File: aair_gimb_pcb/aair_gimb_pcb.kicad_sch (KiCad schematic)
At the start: 0 parts

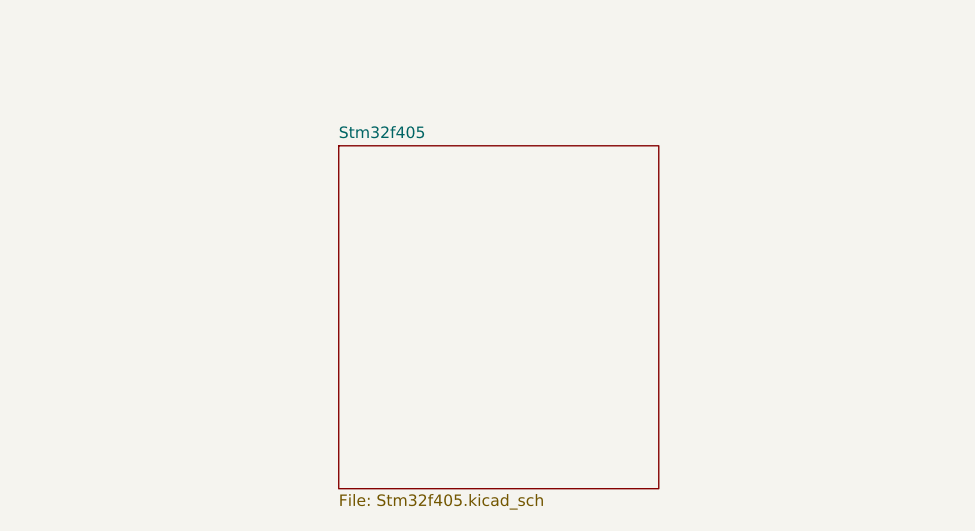
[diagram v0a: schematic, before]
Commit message: macros
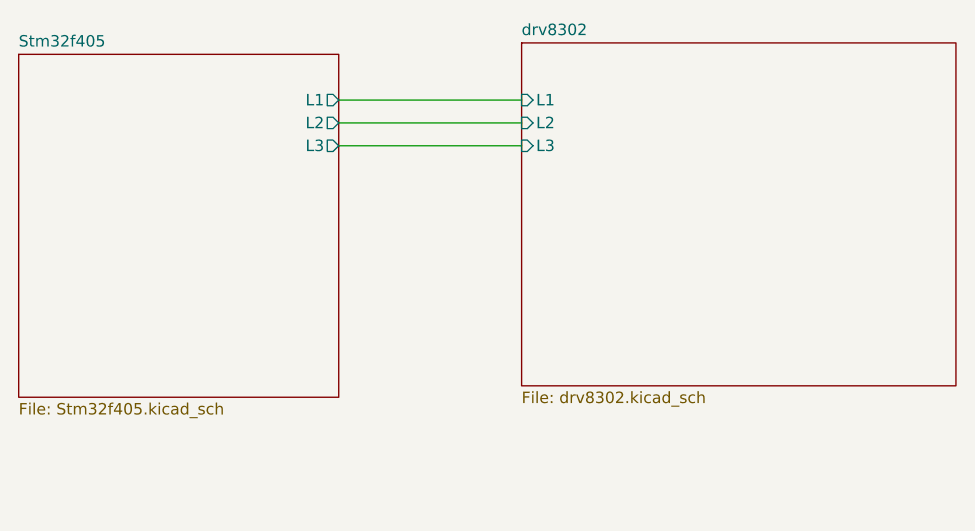
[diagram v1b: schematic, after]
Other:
- added sheet drv8302 (drv8302.kicad_sch)
- sheet Stm32f405 ports: added L1, L2, L3; removed none
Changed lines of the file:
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@@
 	(generator_version "9.0")
 	(paper "A4")
+	(wire
+		(pts
+			(xy 124.46 87.63) (xy 144.78 87.63)
+		)
+		(stroke
+			(width 0)
+			(type default)
+		)
+	)
+	(wire
+		(pts
+			(xy 124.46 85.09) (xy 144.78 85.09)
+		)
+		(stroke
+			(width 0)
+			(type default)
+		)
+	)
+	(wire
+		(pts
+			(xy 124.46 82.55) (xy 144.78 82.55)
+		)
+		(stroke
+			(width 0)
+			(type default)
+		)
+	)
 	(sheet
-		(at 124.46 87.63)
+		(at 144.78 76.2)
+		(size 48.26 38.1)
+		(exclude_from_sim no)
+		(in_bom yes)
+		(on_board yes)
+		(dnp no)
+		(fields_autoplaced yes)
+		(stroke
+			(width 0.1524)
+			(type solid)
+		)
+		(fill
+			(color 0 0 0 0.0000)
+		)
+		(property "Sheetname" "drv8302"
+			(at 144.78 75.4884 0)
+			(effects
+				(font
+					(size 1.27 1.27)
+				)
+				(justify left bottom)
+			)
+		)
+		(property "Sheetfile" "drv8302.kicad_sch"
+			(at 144.78 114.8846 0)
+			(effects
+				(font
+					(size 1.27 1.27)
+				)
+				(justify left top)
+			)
+		)
+		(pin "L3" input
+			(at 144.78 87.63 180)
+			(effects
+				(font
+					(size 1.27 1.27)
+				)
+				(justify left)
+			)
+		)
+		(pin "L2" input
+			(at 144.78 85.09 180)
+			(effects
+				(font
+					(size 1.27 1.27)
+				)
+				(justify left)
+			)
+		)
+		(pin "L1" input
+			(at 144.78 82.55 180)
+			(effects
+				(font
+					(size 1.27 1.27)
+				)
+				(justify left)
+			)
+		)
+		(instances
+			(project "aair_gimb_pcb"
+				(path "/d04c5395-2e3c-40b8-8677-11fb81ced555"
+					(page "3")
+				)
+			)
+		)
+	)
+	(sheet
+		(at 88.9 77.47)
 		(size 35.56 38.1)
 		(exclude_from_sim no)
@@
 		)
 		(property "Sheetname" "Stm32f405"
-			(at 124.46 86.9184 0)
+			(at 88.9 76.7584 0)
 			(effects
 				(font
@@
 		)
 		(property "Sheetfile" "Stm32f405.kicad_sch"
-			(at 124.46 126.3146 0)
+			(at 88.9 116.1546 0)
 			(effects
 				(font
@@
 			)
 		)
+		(pin "L3" output
+			(at 124.46 87.63 0)
+			(effects
+				(font
+					(size 1.27 1.27)
+				)
+				(justify right)
+			)
+		)
+		(pin "L2" output
+			(at 124.46 85.09 0)
+			(effects
+				(font
+					(size 1.27 1.27)
+				)
+				(justify right)
+			)
+		)
+		(pin "L1" output
+			(at 124.46 82.55 0)
+			(effects
+				(font
+					(size 1.27 1.27)
+				)
+				(justify right)
+			)
+		)
